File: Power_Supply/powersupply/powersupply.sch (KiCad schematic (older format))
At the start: 70 parts, among them J1 Conn_01x03, J2 USB_B_Micro, J3 1x2, J4 1x2, Q1 Q_PMOS_GDS, SW1 KMR2, U1 AZ1117E-3.3, U10 INA199, U2 ATSAMD10D13A-SS, U3 B0505S-2WR2, U5 joystick-K1-1506DN-01, U6 MC33063AP1, U7 LM358P

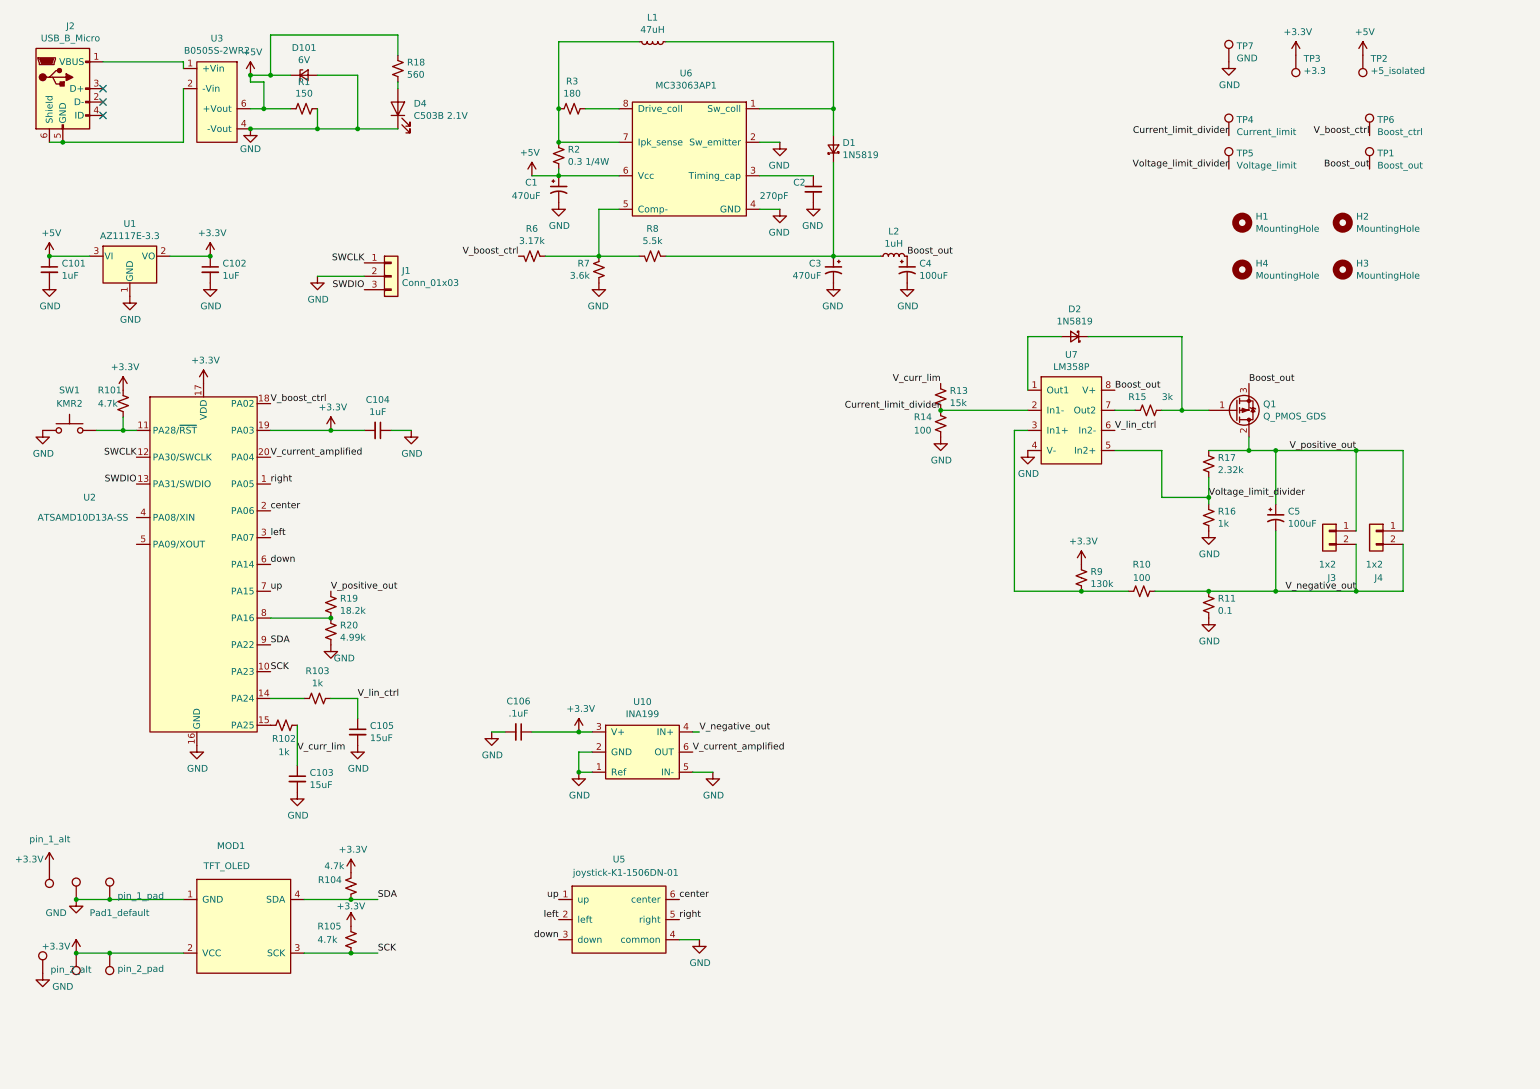
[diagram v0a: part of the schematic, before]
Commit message: small changes
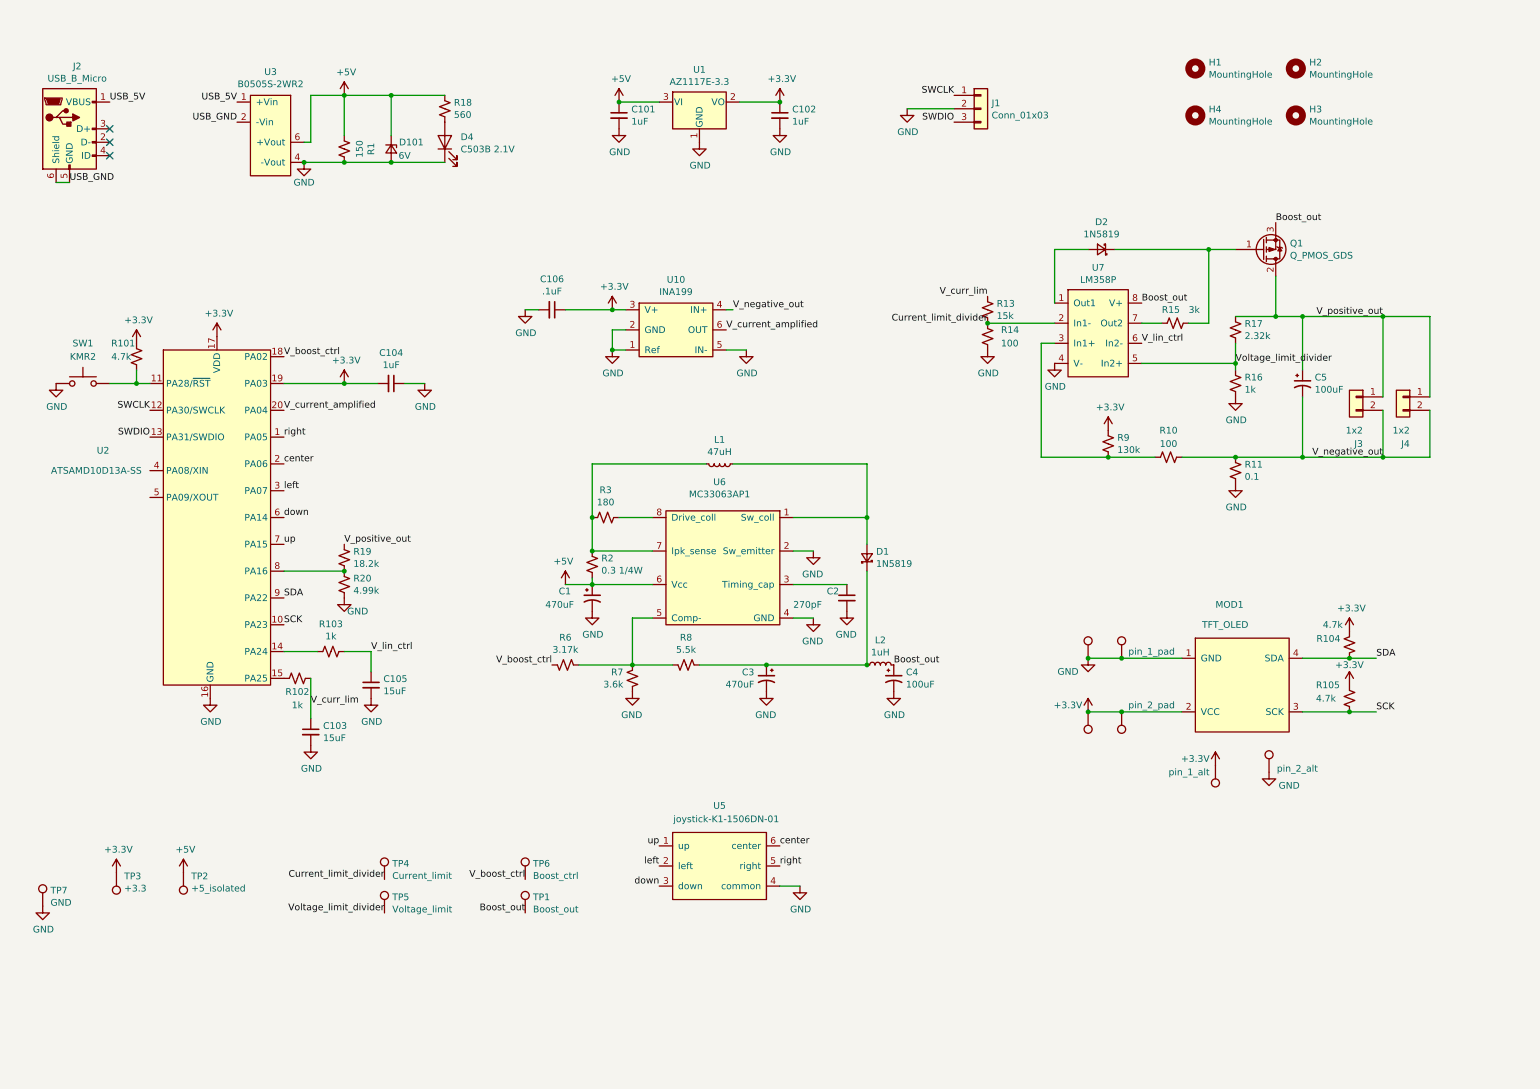
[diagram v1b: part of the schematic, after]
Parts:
- TP13: value TestPoint -> pin_2_pad_alt
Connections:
- net USB_5V: now reaches J2.1 (VBUS), U3.1 (+Vin)
- net USB_GND: now reaches J2.5 (GND), J2.6 (Shield), U3.2 (-Vin)
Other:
- moved on the sheet: C1, C101, C102, C103, C104, C105, C106, C2, C3, C4, C5, D1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
